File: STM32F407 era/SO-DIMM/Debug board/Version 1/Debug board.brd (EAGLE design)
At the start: 91.4 x 33.3 mm, 16 parts, among them J4 FTDI_DEVICE, J8 22-27-2021-02, X1 057-014-1, X2 BN35N61, X3 BN35N61, X4 BN35N61, X5 BN35N61, X6 BN35N61

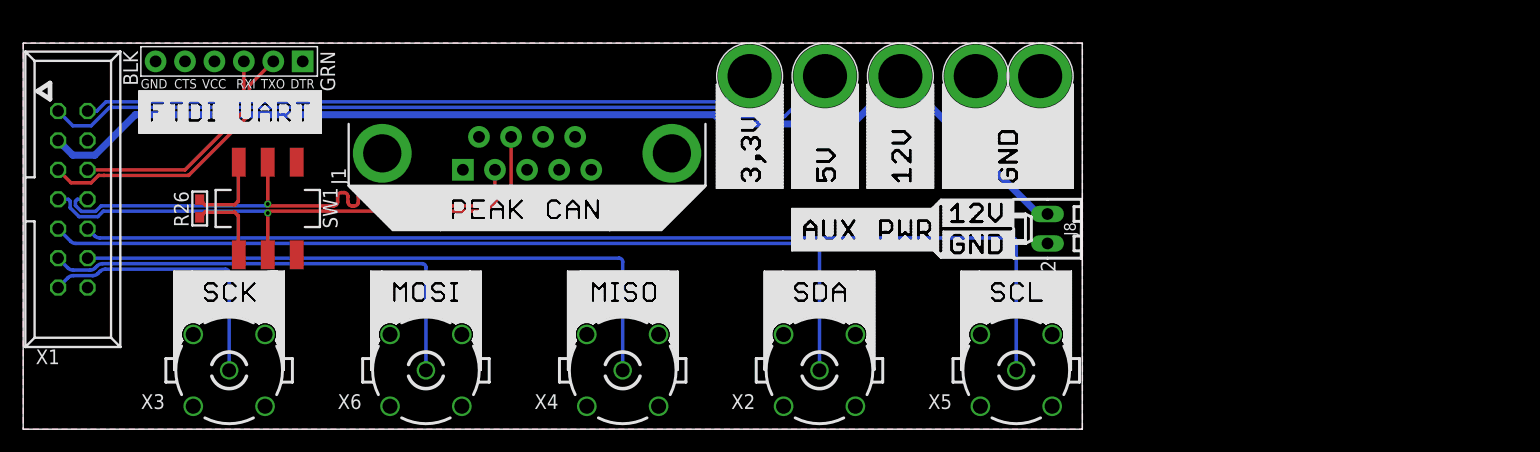
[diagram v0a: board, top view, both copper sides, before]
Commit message: All board V1-RC1 done
all boards ready for inspection
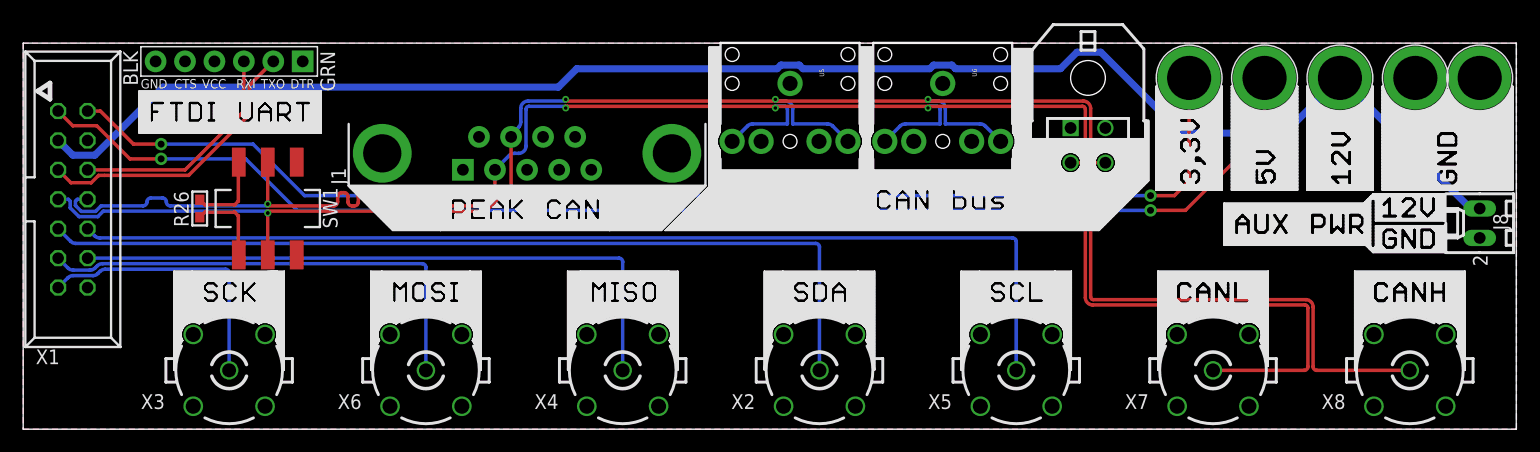
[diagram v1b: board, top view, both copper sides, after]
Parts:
- added U$21: MICROFIT4, unicorn:43045-0400
- added U5, U6: (no value), connector:AUDIO-JACK
- added X7, X8: BN35N61, con-coax:B35N61
- moved J7 37.9 mm to (125.6, 38.6)
- moved J2 37.9 mm to (100.5, 38.6)
- moved J3 37.9 mm to (107.0, 38.6)
- moved J5 37.9 mm to (113.5, 38.6)
- moved J6 37.9 mm to (120.0, 38.6)
- moved J8 37.3 mm to (125.6, 26.0)
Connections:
- net CAN_N: now also U$21.P$3, U5.TIP, U6.TIP, X7.1
- net CAN_P: now also U$21.P$4, U5.RING, U6.RING, X8.1
- net GND: now also U$21.P$1, U$21.P$2, U5.SLEEVE, U6.SLEEVE, X7.2, X7.3, X7.4, X7.5, X8.2, X8.3, X8.4, X8.5
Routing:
- net CAN_N: track 49.1 -> 172.2 mm, vias 1 -> 4
- net CAN_P: track 50.3 -> 171.2 mm, vias 1 -> 4
- net 3.3V: track 58.4 -> 107.5 mm, vias 0 -> 2
- net 5.0V: track 69.2 -> 115.1 mm, vias 0 -> 2
- net 12V: track 94.4 -> 137.0 mm
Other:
- board size 91.4 x 33.3 mm -> 128.9 x 33.3 mm
